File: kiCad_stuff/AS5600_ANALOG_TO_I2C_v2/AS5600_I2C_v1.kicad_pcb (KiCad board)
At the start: 2 copper layers, 25 x 17 mm, 10 parts, among them J1 Conn_01x04, U2 MCP3221

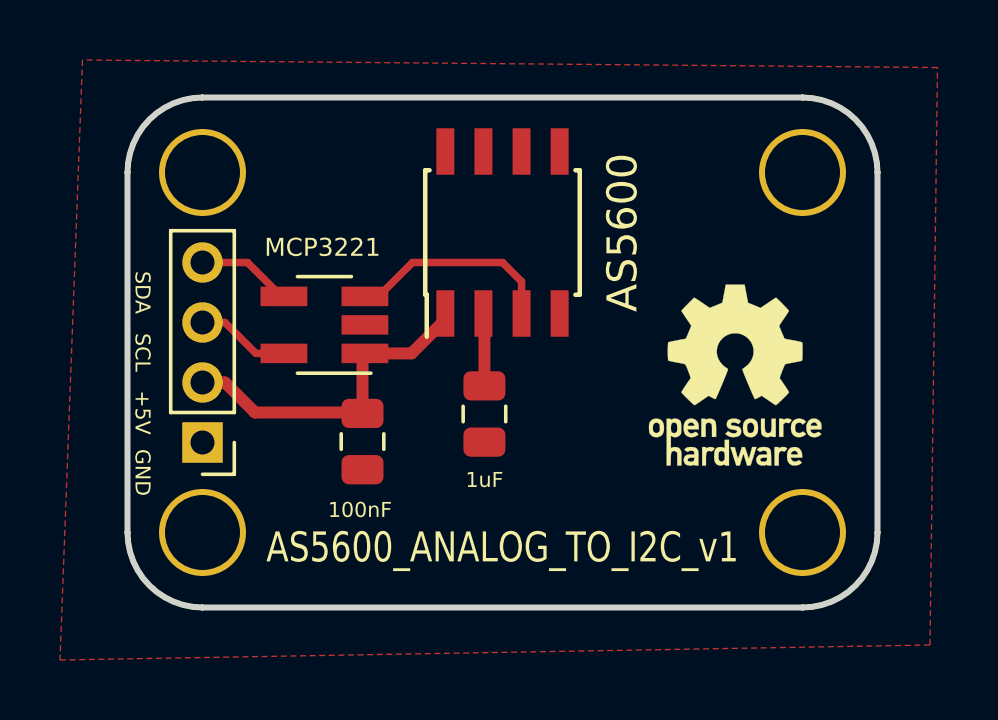
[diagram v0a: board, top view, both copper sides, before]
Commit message: some minor tweaks
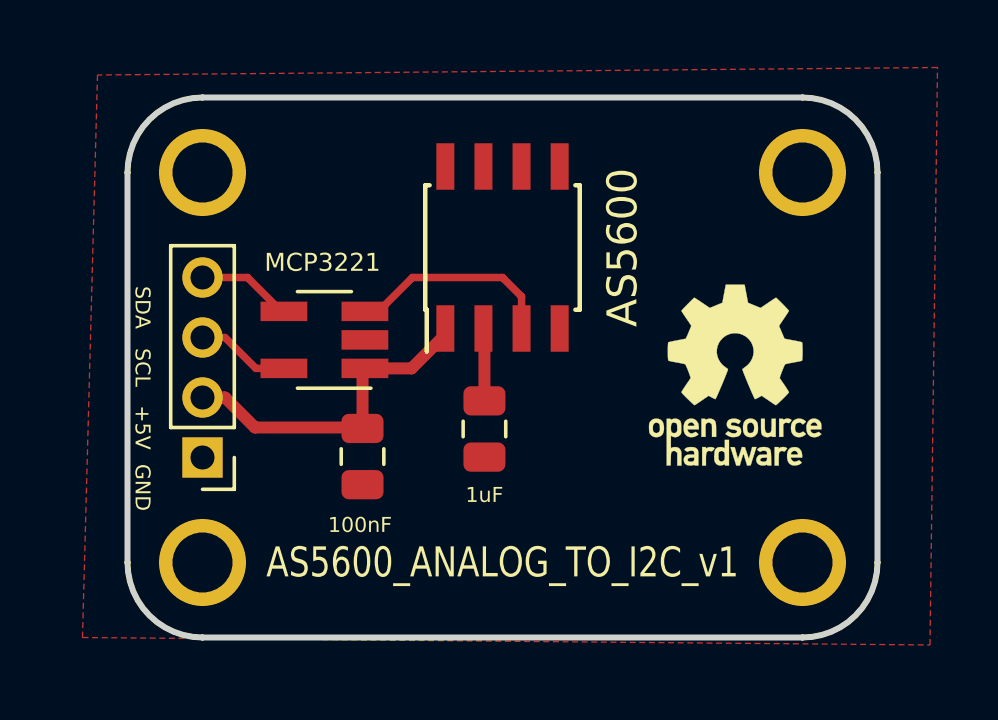
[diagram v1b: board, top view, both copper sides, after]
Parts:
- moved 2.5mm  1.00 mm to (172.0, 74.0)
- moved 2.5mm  1.00 mm to (152.0, 74.0)
- moved AS5600 0.50 mm to (162.0, 61.5)
- moved C1 0.50 mm to (157.3, 68.5)
- moved C2 0.50 mm to (161.4, 67.5)
- moved J1 0.50 mm to (152.0, 68.5)
- moved U2 0.50 mm to (156.1, 64.6)
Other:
- board size 25 x 17 mm -> 25 x 18 mm
